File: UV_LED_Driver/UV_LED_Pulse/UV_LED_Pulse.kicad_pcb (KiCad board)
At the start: 2 copper layers, 36 x 18 mm, 30 parts, among them J1 PWR/Signal, Q1 BC817, Q2 2N7002

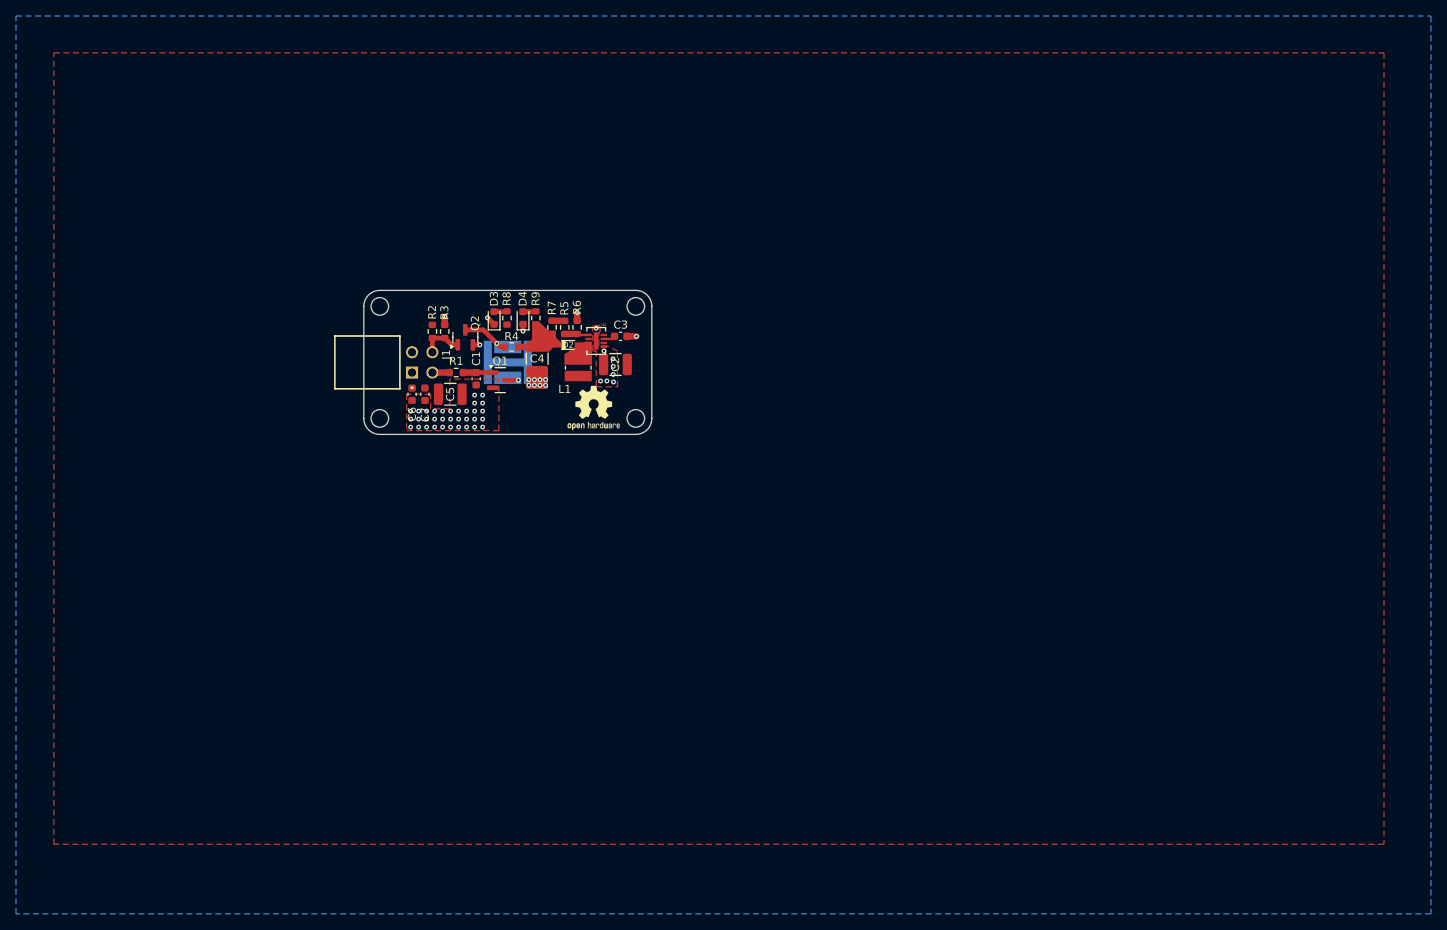
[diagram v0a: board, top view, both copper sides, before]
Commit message: .
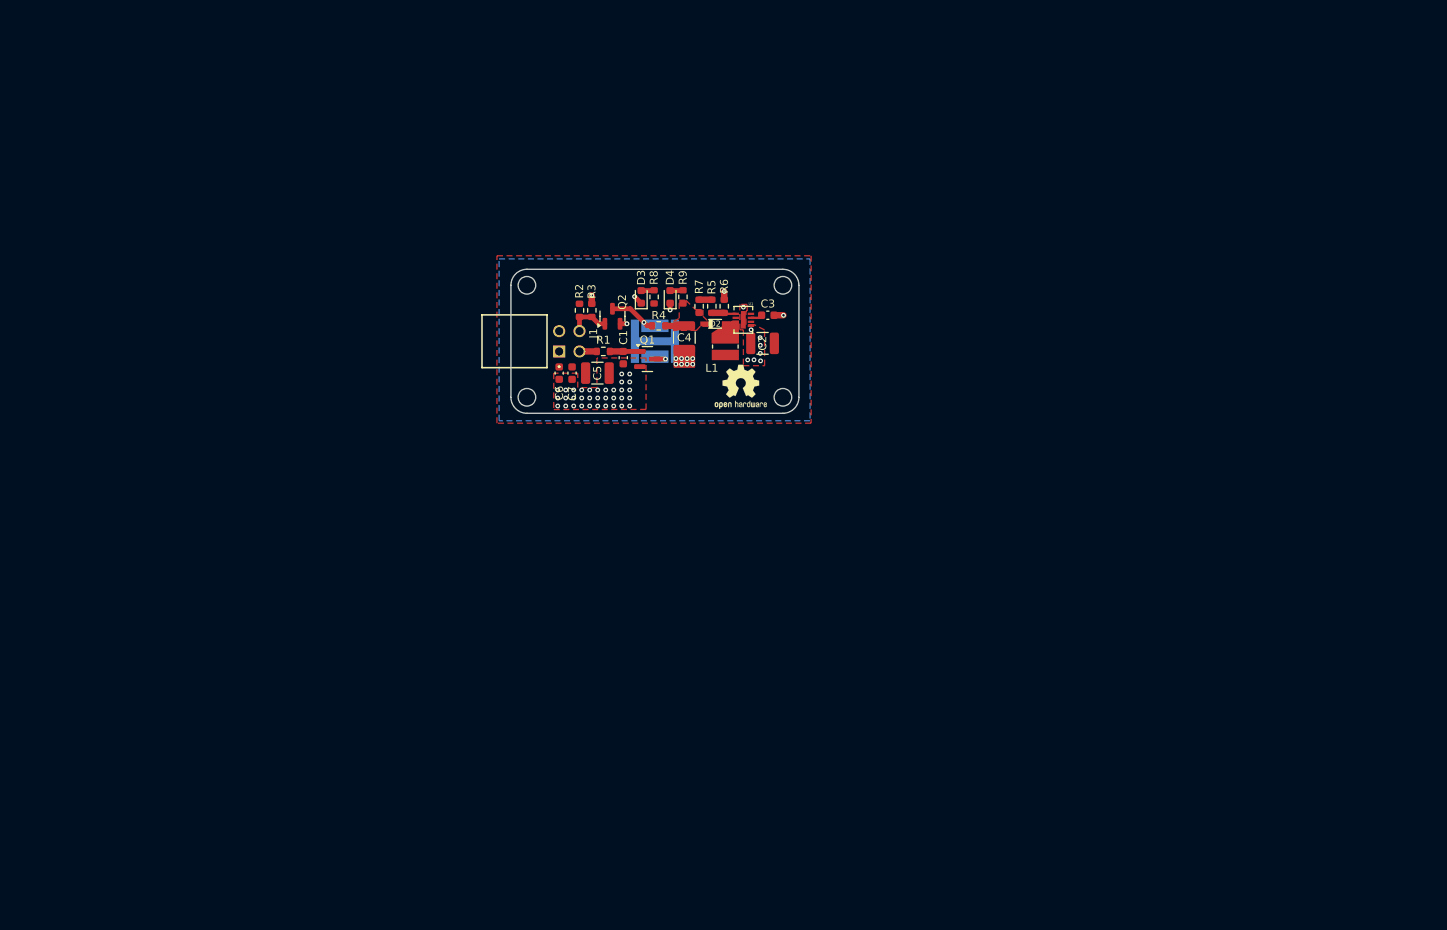
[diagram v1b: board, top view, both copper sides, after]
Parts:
- moved C1 18.6 mm to (101.1, 71.3)
- moved C3 18.6 mm to (119.2, 66.0)
- moved C5 18.6 mm to (97.8, 73.2)
- moved D1 18.6 mm to (105.0, 69.3)
- moved D2 18.6 mm to (112.6, 67.1)
- moved D3 18.6 mm to (103.3, 63.7)
- moved D4 18.6 mm to (106.9, 63.7)
- moved Q1 18.6 mm to (104.1, 71.5)
- moved R2 18.6 mm to (95.6, 65.4)
- moved R5 18.6 mm to (112.2, 64.9)
- moved R6 18.6 mm to (113.7, 64.9)
- moved R7 18.6 mm to (110.6, 64.9)
- moved REF** 18.6 mm to (121.0, 76.3)
- moved REF** 18.6 mm to (89.0, 62.3)
- moved REF** 18.6 mm to (89.0, 76.3)
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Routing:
- added copper zone on F.Cu, net 5.8V
